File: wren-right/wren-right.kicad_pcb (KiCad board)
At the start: 2 copper layers, 93 parts, among them J1 TRRS_Jack, SW0 Reset, U1 ProMicro

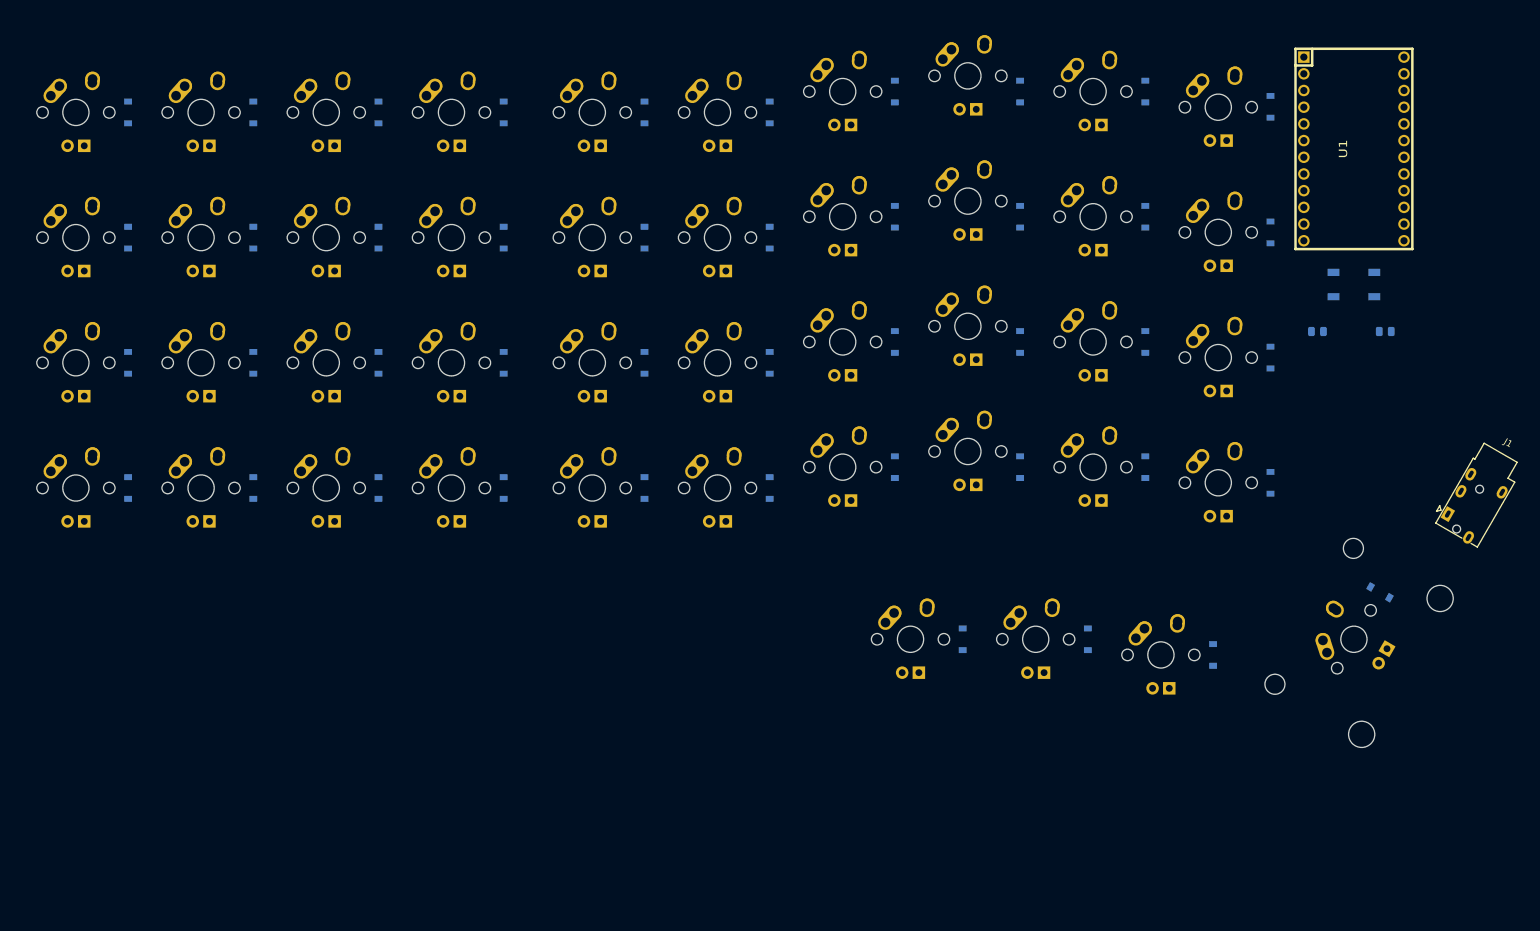
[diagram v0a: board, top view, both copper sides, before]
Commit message: Tracks Finished
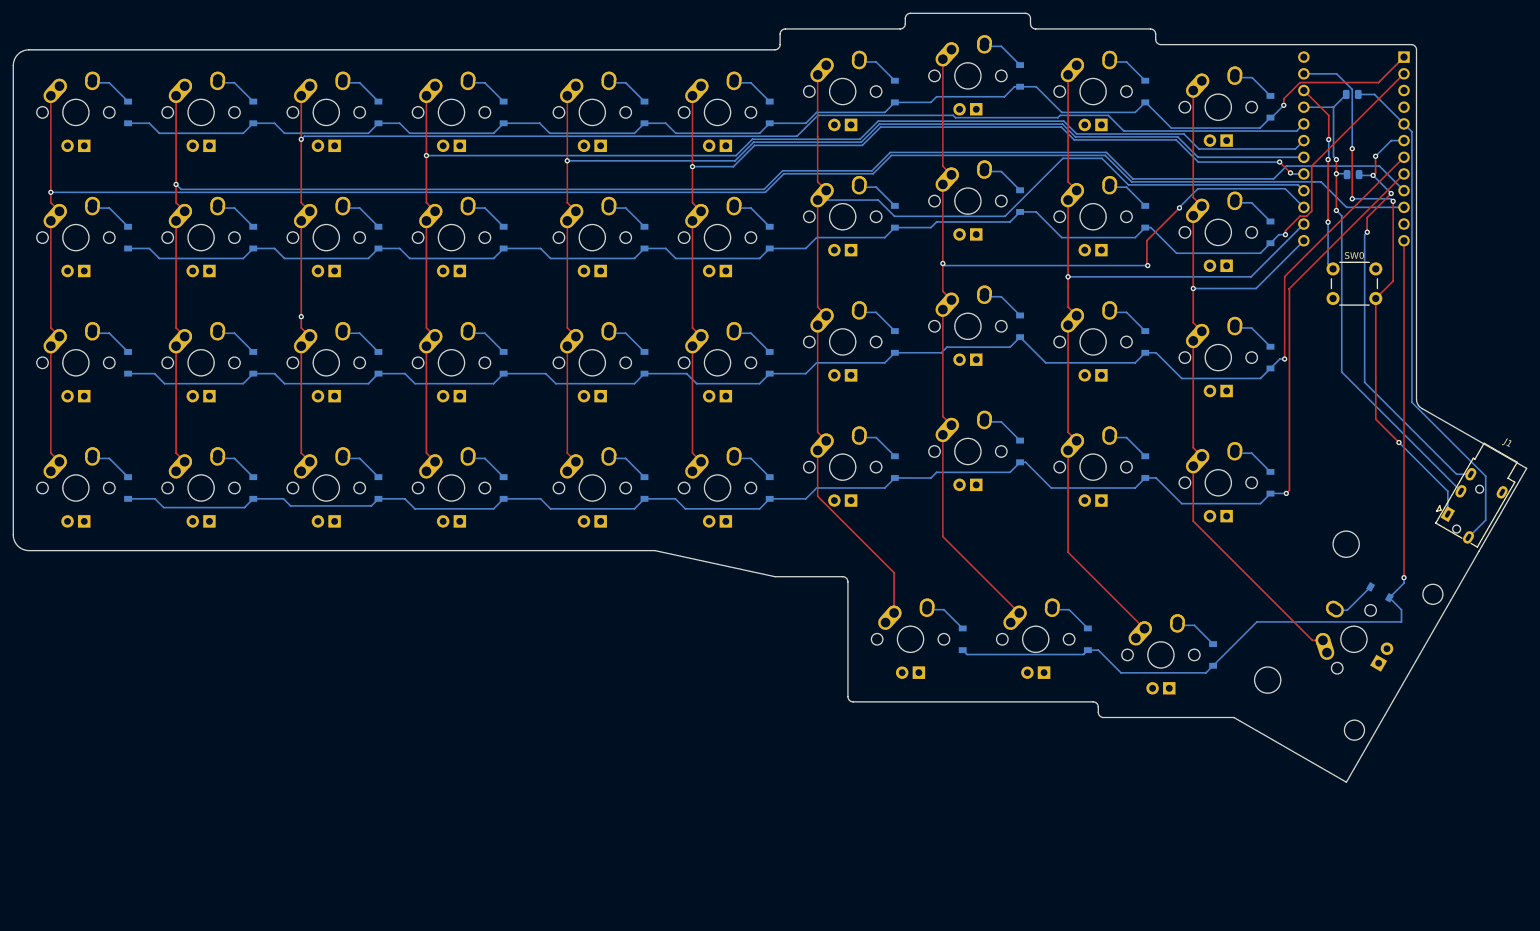
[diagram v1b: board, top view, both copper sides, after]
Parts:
- MX41: footprint MX_Only:MX-2U -> MX_Only:MX-2U-FLIPPED-ReversedStabilizers
- SW0: footprint random-keyboard-parts:SKQG-1155865 -> Button_Switch_THT:SW_PUSH_6mm; moved to F.Cu
- U1: moved to B.Cu
- moved R1 36.4 mm to (241.0, 33.8)
- moved R2 24.5 mm to (241.2, 46.0)
- moved SW0 3.97 mm to (238.1, 60.3)
- moved D13 2.38 mm to (190.5, 50.0)
- moved D3 2.38 mm to (190.5, 31.0)
- moved D23 2.38 mm to (190.5, 69.1)
- moved D33 2.38 mm to (190.5, 88.1)
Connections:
- U1 pad 1: COL8 -> ROW0
- U1 pad 10: ROW3 -> COL9
- U1 pad 11: ROW4 -> Net-(U1-Pad11)
- U1 pad 12: Net-(U1-Pad12) -> ROW4
- U1 pad 13: COL7 -> COL0
- U1 pad 14: COL6 -> COL1
- U1 pad 15: COL5 -> COL2
- U1 pad 16: COL4 -> COL3
- U1 pad 17: COL3 -> COL4
- U1 pad 18: COL2 -> COL5
- U1 pad 19: COL1 -> COL6
- U1 pad 2: COL9 -> ROW1
- U1 pad 20: COL0 -> COL7
- U1 pad 7: ROW0 -> ROW2
- U1 pad 8: ROW1 -> ROW3
- U1 pad 9: ROW2 -> COL8
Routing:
- net COL9: track 0.00 -> 265.9 mm, vias 0 -> 1
- net COL8: track 0.00 -> 247.9 mm, vias 0 -> 1
- net ROW3: track 0.00 -> 244.9 mm, vias 0 -> 1
- net ROW2: track 0.00 -> 227.9 mm, vias 0 -> 1
- net ROW1: track 0.00 -> 222.3 mm, vias 0 -> 1
- net ROW0: track 0.00 -> 211.7 mm, vias 0 -> 1
- net COL7: track 0.00 -> 210.2 mm, vias 0 -> 2
- net COL6: track 0.00 -> 192.4 mm, vias 0 -> 1
- net COL5: track 0.00 -> 170.9 mm, vias 0 -> 1
- net COL3: track 0.00 -> 164.6 mm
- net COL4: track 0.00 -> 152.9 mm, vias 0 -> 3
- net COL2: track 0.00 -> 149.9 mm, vias 0 -> 3
- net ROW4: track 0.00 -> 131.7 mm, vias 0 -> 1
- net COL1: track 0.00 -> 125.5 mm, vias 0 -> 1
- net COL0: track 0.00 -> 109.9 mm, vias 0 -> 1
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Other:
- board outline added: 230.3 x 117 mm

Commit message: Left Side Finished
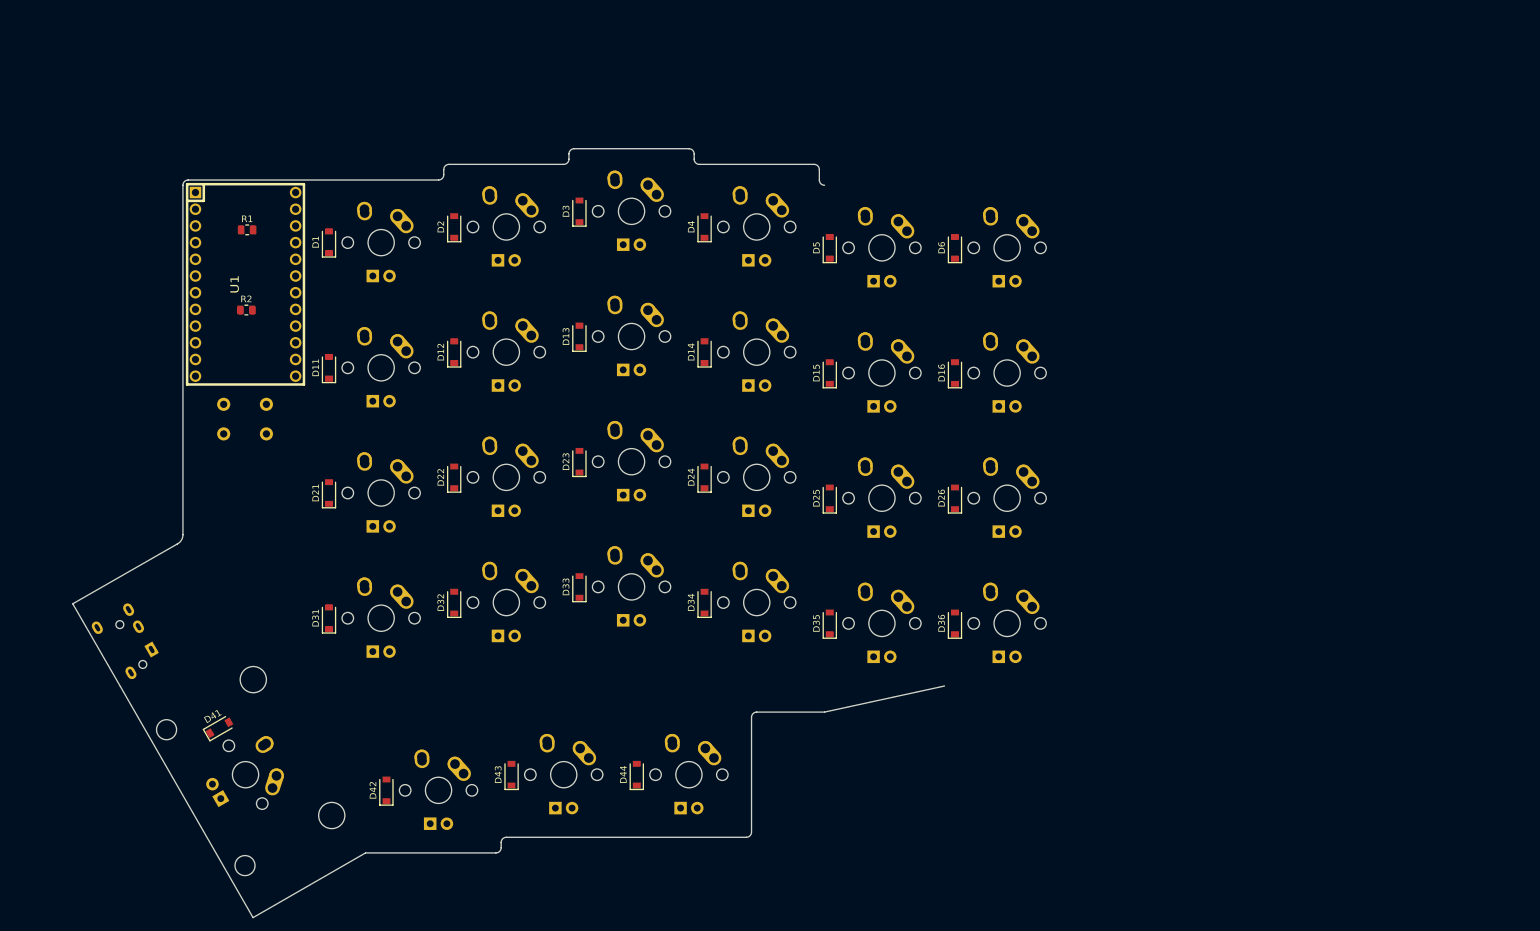
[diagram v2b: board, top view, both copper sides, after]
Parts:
- removed D10, D17, D18, D19, D20, D27, D28, D29, D30, D37, D38, D39, D40, D7, D8, D9: D_Small, Diode_SMD:D_SOD-123
- removed MX10, MX17, MX18, MX19, MX20, MX27, MX28, MX29, MX30, MX37, MX38, MX39, MX40, MX7, MX8, MX9: MX-NoLED, MX_Only:MX-1U
- D1, D11, D12, D13, D14, D15, D16, D2, D21, D22, D23, D24, D25, D26, D3, D31, D32, D33, D34, D35, D36, D4, D41, D42, D43, D44, D5, D6, R1, R2, U1: moved to F.Cu
- J1, MX1, MX11, MX12, MX13, MX14, MX15, MX16, MX2, MX21, MX22, MX23, MX24, MX25, MX26, MX3, MX31, MX32, MX33, MX34, MX35, MX36, MX4, MX41, MX42, MX43, MX44, MX5, MX6, SW0: moved to B.Cu
- moved J1 198.3 mm to (58.4, 118.2), turned to 210 degrees
- moved D41 177.8 mm to (68.7, 130.1), turned to 30 degrees
- moved MX41 169.9 mm to (72.6, 137.3), turned to 120 degrees
- moved U1 169.9 mm to (72.6, 62.7)
- moved R2 169.7 mm to (72.8, 66.6), turned to 0 degrees
- moved R1 169.4 mm to (72.9, 54.4), turned to 0 degrees
- moved SW0 163.6 mm to (75.8, 80.9), turned to 180 degrees
- moved D1 144.7 mm to (85.3, 56.3)
- moved D11 144.7 mm to (85.3, 75.4)
- moved D21 144.7 mm to (85.3, 94.4)
- moved D31 144.7 mm to (85.3, 113.5)
- moved MX1 129.0 mm to (93.3, 56.3), turned to 180 degrees
- moved MX11 129.0 mm to (93.3, 75.4), turned to 180 degrees
- moved MX21 129.0 mm to (93.3, 94.4), turned to 180 degrees
- moved MX31 129.0 mm to (93.3, 113.5), turned to 180 degrees
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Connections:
- U1 pad 10: COL9 -> Net-(U1-Pad10)
- U1 pad 12: ROW4 -> Net-(U1-Pad12)
- U1 pad 19: COL6 -> Net-(U1-Pad19)
- U1 pad 20: COL7 -> Net-(U1-Pad20)
- U1 pad 9: COL8 -> Net-(U1-Pad9)
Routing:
- net COL9: track 265.9 -> 0.00 mm, vias 1 -> 0
- net COL8: track 247.9 -> 0.00 mm, vias 1 -> 0
- net ROW3: track 244.9 -> 0.00 mm, vias 1 -> 0
- net ROW2: track 227.9 -> 0.00 mm, vias 1 -> 0
- net ROW1: track 222.3 -> 0.00 mm, vias 1 -> 0
- net ROW0: track 211.7 -> 0.00 mm, vias 1 -> 0
- net COL7: track 210.2 -> 0.00 mm, vias 2 -> 0
- net COL6: track 192.4 -> 0.00 mm, vias 1 -> 0
- net COL5: track 170.9 -> 0.00 mm, vias 1 -> 0
- net COL3: track 164.6 -> 0.00 mm
- net COL4: track 152.9 -> 0.00 mm, vias 3 -> 0
- net COL2: track 149.9 -> 0.00 mm, vias 3 -> 0
- net ROW4: track 131.7 -> 0.00 mm, vias 1 -> 0
- net COL1: track 125.5 -> 0.00 mm, vias 1 -> 0
- net COL0: track 109.9 -> 0.00 mm, vias 1 -> 0
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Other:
- board size 230.3 x 117 mm -> 132.7 x 117 mm
